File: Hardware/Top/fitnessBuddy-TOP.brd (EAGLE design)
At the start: 38 x 38 mm, 50 parts, among them SW3 SWITCH.MOM, SW4 SWITCH.MOM, U1 NRF52832_MODULE_MDBT42, U2 FT231XS

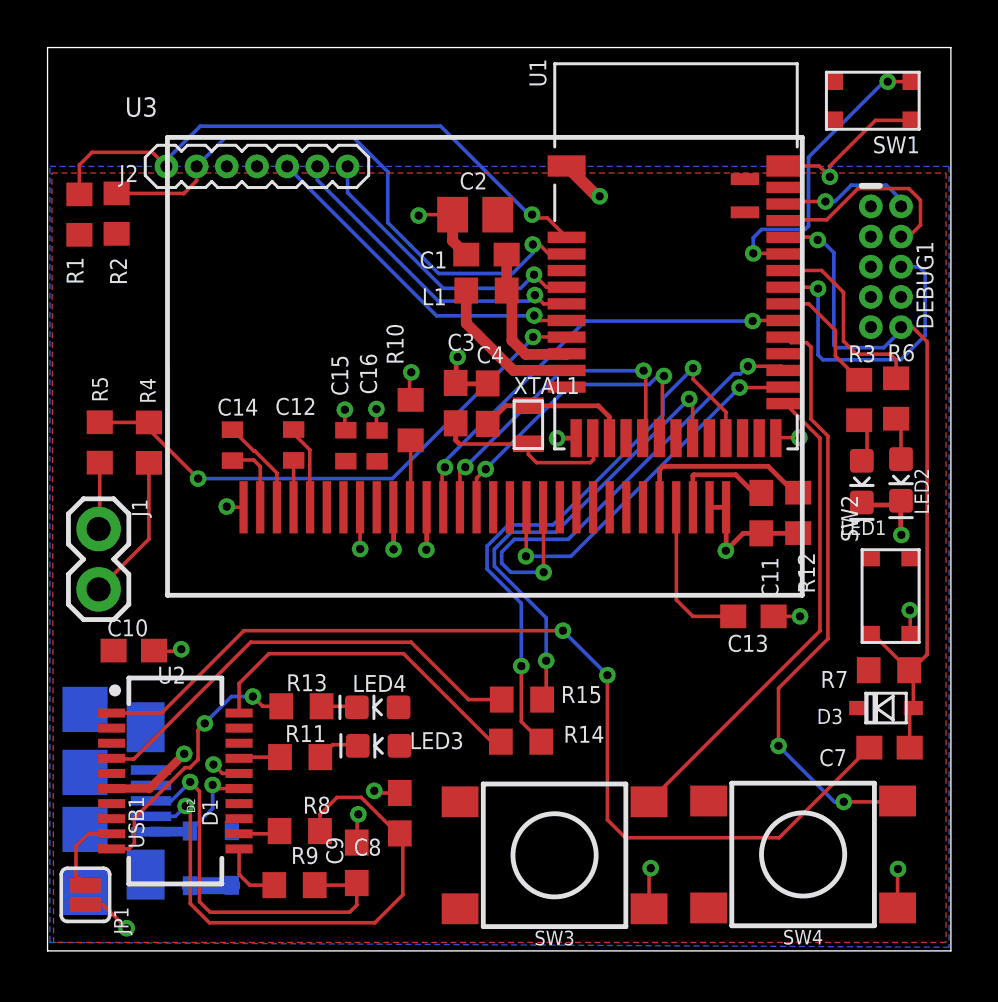
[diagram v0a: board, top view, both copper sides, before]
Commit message: organized top board
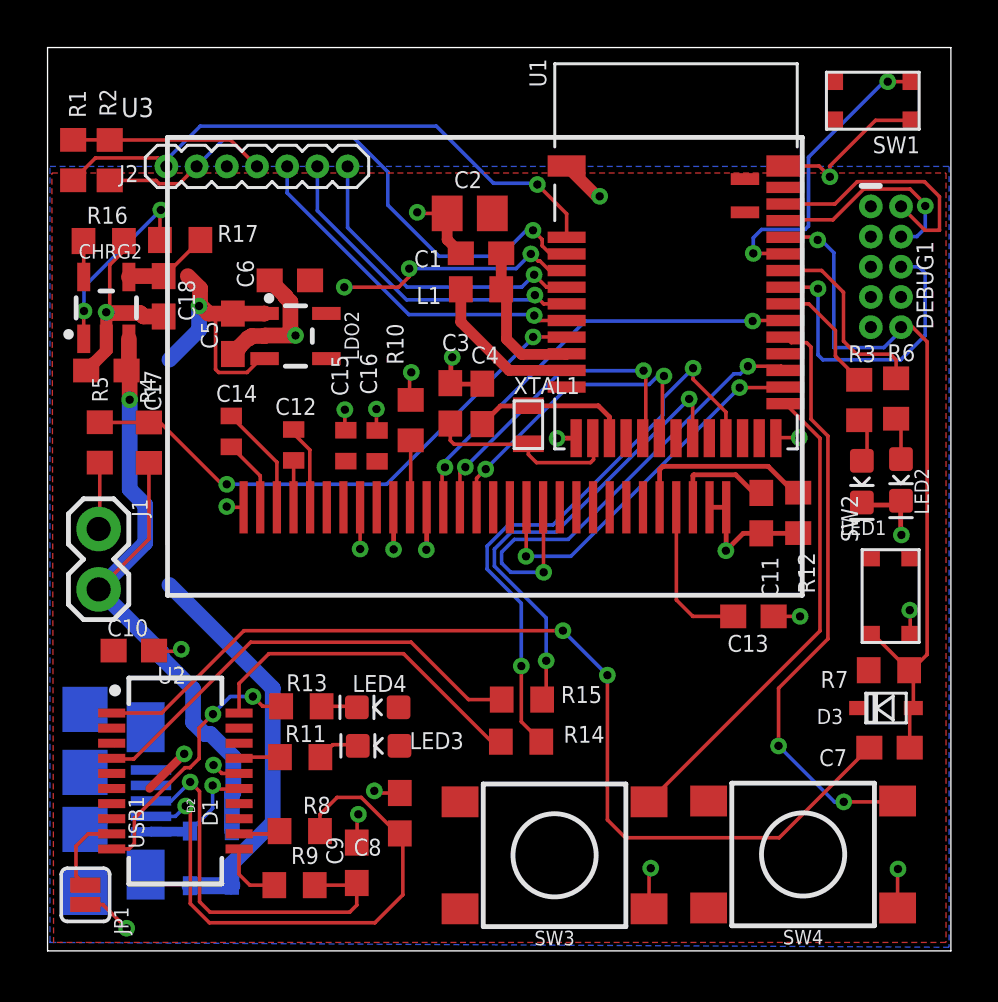
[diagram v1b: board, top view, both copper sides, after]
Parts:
- added C17, C18: 4.7u, LinnesLab-Passives:C0603
- added C5, C6: 1u, LinnesLab-Passives:C0603
- added CHRG2: MCP73831, LinnesLab-Power:SOT23-5
- added LDO2: MIC5504, LinnesLab-Power:SOT23-5
- added R16: (no value), LinnesLab-Passives:R0603
- added R17: 100k, LinnesLab-Passives:R0603
- moved R1 2.31 mm to (1.08, 33.3), turned to 90 degrees
- moved R2 2.27 mm to (2.62, 33.3), turned to 90 degrees
- moved C14 0.58 mm to (7.73, 21.9)
- moved C1 0.23 mm to (18.2, 29.3)
- moved C2 0.23 mm to (17.8, 31.0)
- moved L1 0.23 mm to (18.2, 27.8)
- moved C4 0.23 mm to (18.3, 23.0)
- moved C3 0.23 mm to (16.9, 23.0)
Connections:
- new net N$16: CHRG2.5, R16.2
- new net N$17: C18.2, CHRG2.4, R17.2
- net 3.3V: now also C6.1, LDO2.5
- net D27/CHRG.STATUS: now also CHRG2.1, R17.1
- net GND: now also C17.2, C18.1, C5.1, C6.2, CHRG2.2, LDO2.2, R16.1
- net VIN: now also C5.2, LDO2.1, LDO2.3
- net VLIPO: now also C17.1, CHRG2.3
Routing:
- net VIN: track 1.77 -> 28.9 mm, vias 0 -> 1
- net VLIPO: track 6.20 -> 30.6 mm, vias 0 -> 1
- net D27/CHRG.STATUS: track 0.00 -> 18.5 mm, vias 0 -> 5
- net GND: track 53.7 -> 66.5 mm, vias 25 -> 27
- net 3.3V: track 0.16 -> 8.36 mm
- net SWDIO: track 5.74 -> 10.6 mm, vias 1 -> 0
- net N$17: track 0.00 -> 3.65 mm
- net N$16: track 0.00 -> 1.52 mm
- net SCL: track 24.9 -> 24.0 mm
- net A4/PPG: track 12.4 -> 13.3 mm
- net A5/TIA: track 13.4 -> 14.1 mm
- net D30/LED.CTRL: track 14.5 -> 15.1 mm
- net N$5: track 4.06 -> 4.64 mm
- net SWCLK: track 8.51 -> 8.87 mm, vias 0 -> 1
